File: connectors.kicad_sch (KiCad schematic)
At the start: 16 parts, among them J3 5747841-4, J4 5747841-4

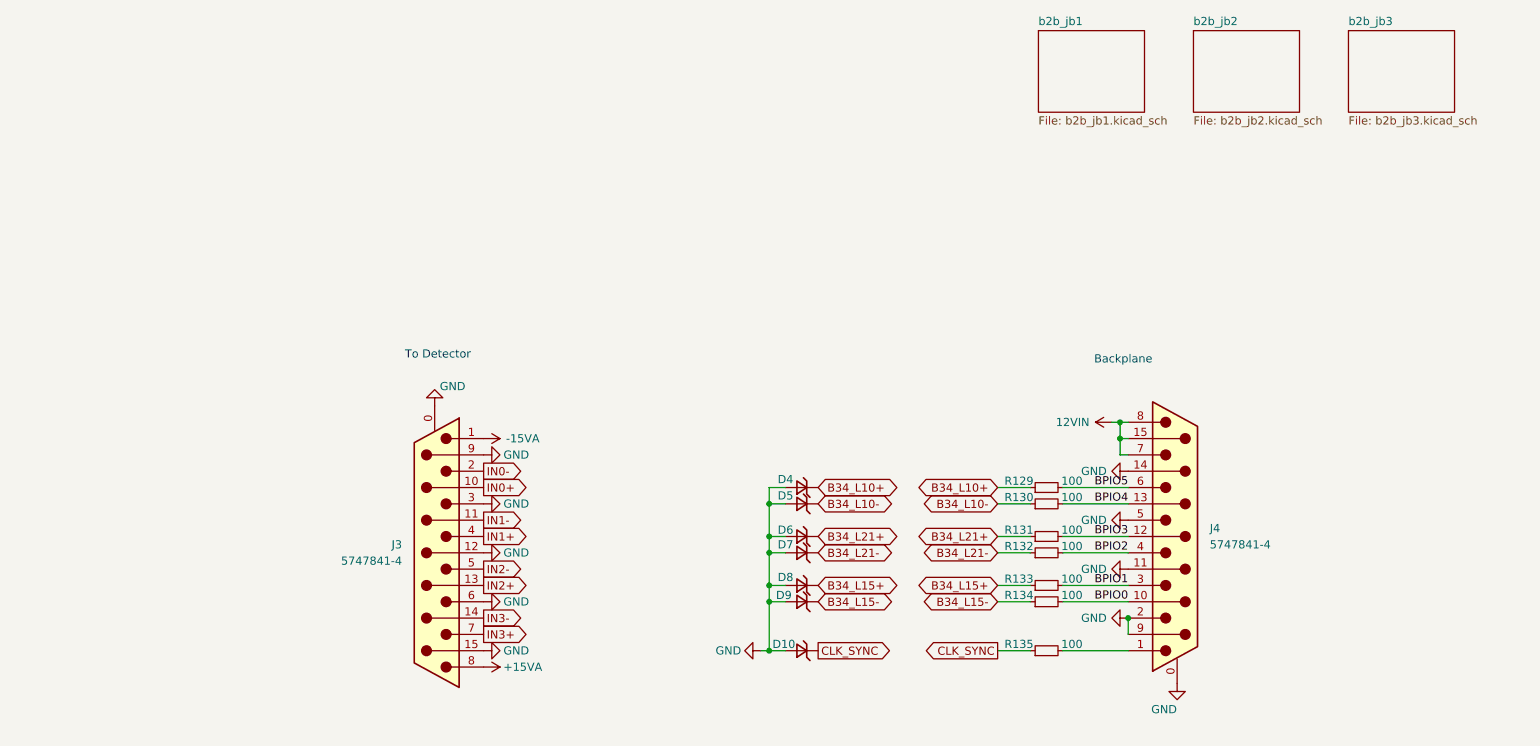
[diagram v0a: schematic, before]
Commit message: Major schematic and PCB changes and latex manual creation.
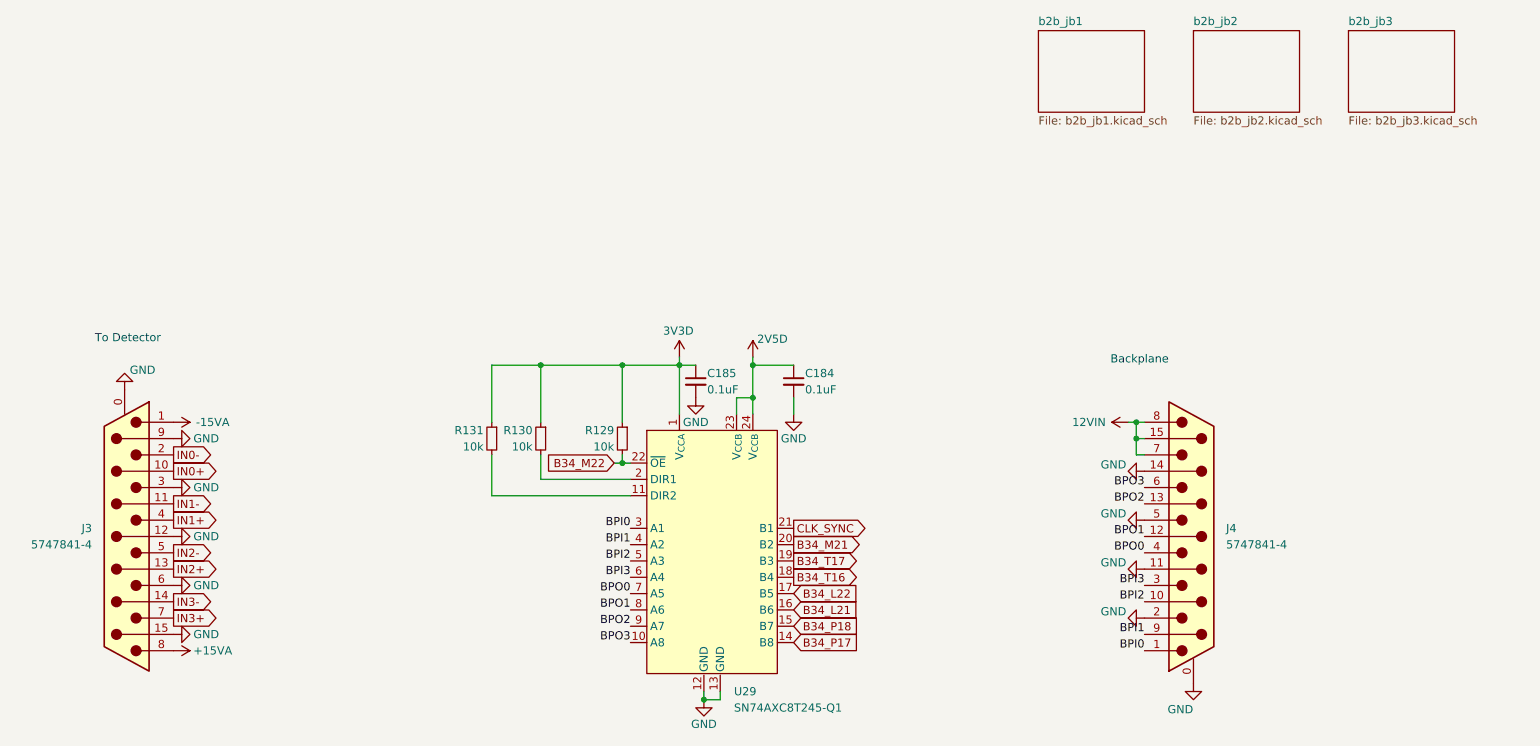
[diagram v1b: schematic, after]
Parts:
- removed D10, D4, D5, D6, D7, D8, D9: ~, lib:TVS_0402_1005Metric, symbol lib:uni_tvs
- removed R132, R133, R134, R135: 100, Resistor_SMD:R_0402_1005Metric, symbol Device:R_Small
- added C184, C185: 0.1uF, Capacitor_SMD:C_0402_1005Metric, symbol Device:C_Small
- added U29: SN74AXC8T245-Q1, Package_SO:TSSOP-24_4.4x7.8mm_P0.65mm, symbol lib:SN74AXC8T245-Q1
- R129, R130, R131: value 100 -> 10k; footprint Resistor_SMD:R_0402_1005Metric -> Resistor_SMD:R_0603_1608Metric; MPN CRCW0402100RFKEDHP -> CRCW060310K0FKEA
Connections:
- net B34_L10- is gone; now on net 3V3D: R130.1
- net B34_L21+ is gone; now on net 3V3D: R131.1
- net CLK_SYNC: now also U29.21 (B1)
- net GND: now also C184.2, C185.2, U29.12 (GND), U29.13 (GND); no longer J4.9 (P9)
- net BPI0: now reaches J4.1
- net BPI0: now also U29.3 (A1)
- net B34_L10+ renamed 3V3D
- net 3V3D: now also C185.1, U29.1 (V_{CCA})
- net BPIO0 renamed BPI2
- net BPI2: now also U29.5 (A3)
- net BPIO1 renamed BPI3
- net BPI3: now also U29.6 (A4)
- net BPIO2 renamed BPO0
- net BPO0: now also U29.7 (A5)
- net BPIO3: no longer names the net of R131.2
- net BPIO3: now also U29.11 (DIR2); no longer J4.12 (P12)
- net BPIO4: no longer names the net of R130.2
- net BPIO4: now also U29.2 (DIR1); no longer J4.13 (P13)
- net BPIO5 renamed B34_M22
- net B34_M22: now also U29.22 (~{OE}); no longer J4.6
- new net 2V5D: C184.1, U29.23 (V_{CCB}), U29.24 (V_{CCB})
- new net B34_L21: U29.16 (B6)
- new net B34_L22: U29.17 (B5)
- new net B34_M21: U29.20 (B2)
- new net B34_P17: U29.14 (B8)
- new net B34_P18: U29.15 (B7)
- new net B34_T16: U29.18 (B4)
- new net B34_T17: U29.19 (B3)
- new net BPI1: J4.9 (P9), U29.4 (A2)
- new net BPO1: J4.12 (P12), U29.8 (A6)
- new net BPO2: J4.13 (P13), U29.9 (A7)
- new net BPO3: J4.6, U29.10 (A8)
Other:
- moved on the sheet: J3, J4
